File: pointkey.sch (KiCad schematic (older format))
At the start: 12 parts, among them P1 CONN_01X02, SW1 SW_PUSH, SW2 SW_PUSH, U1 4013

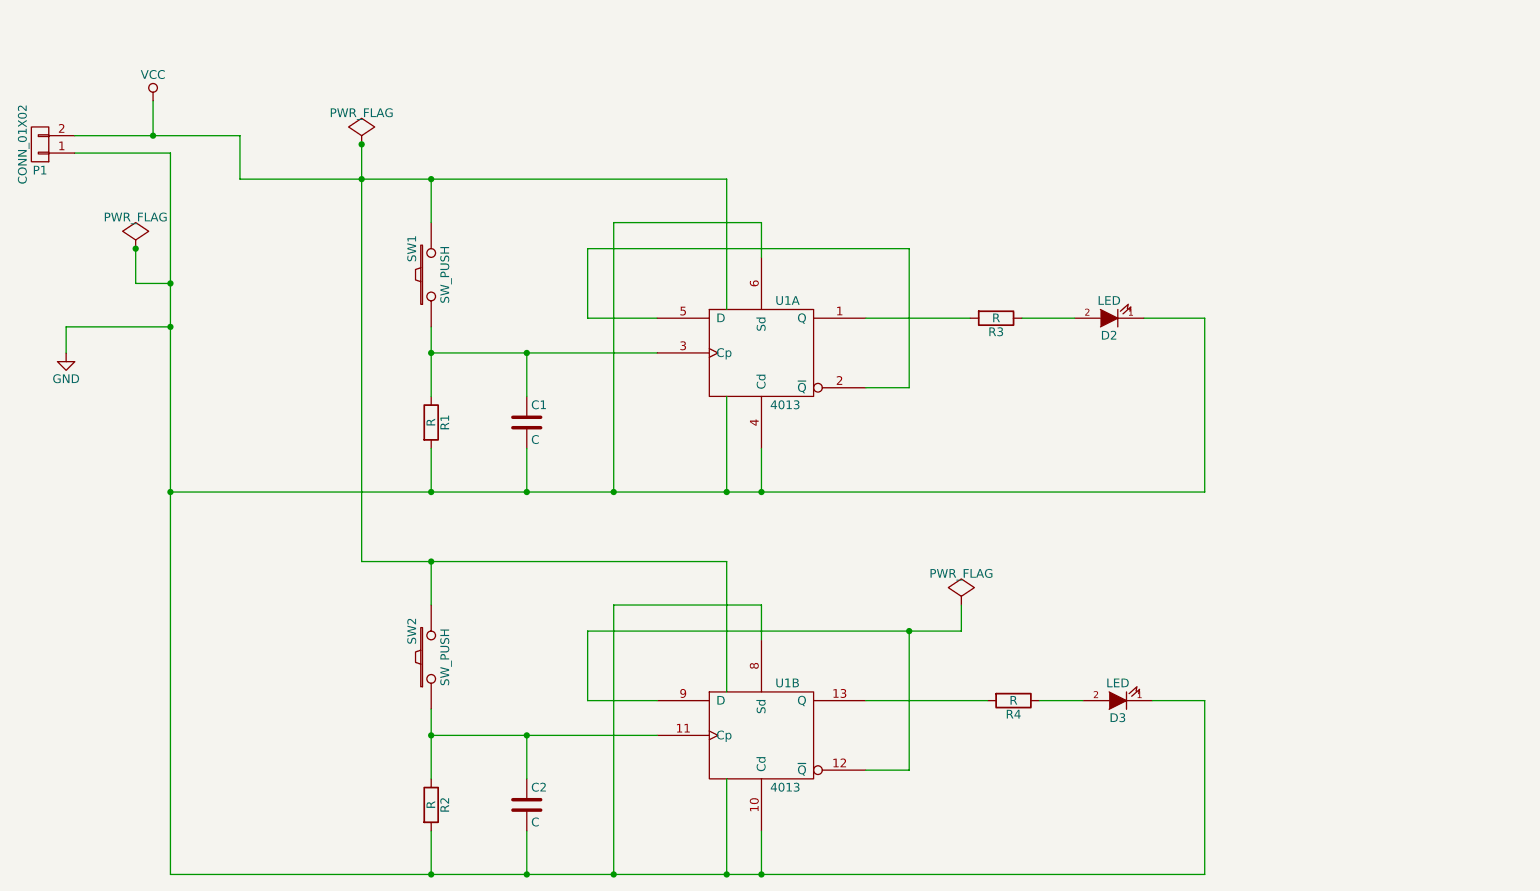
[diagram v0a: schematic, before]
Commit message: debounce
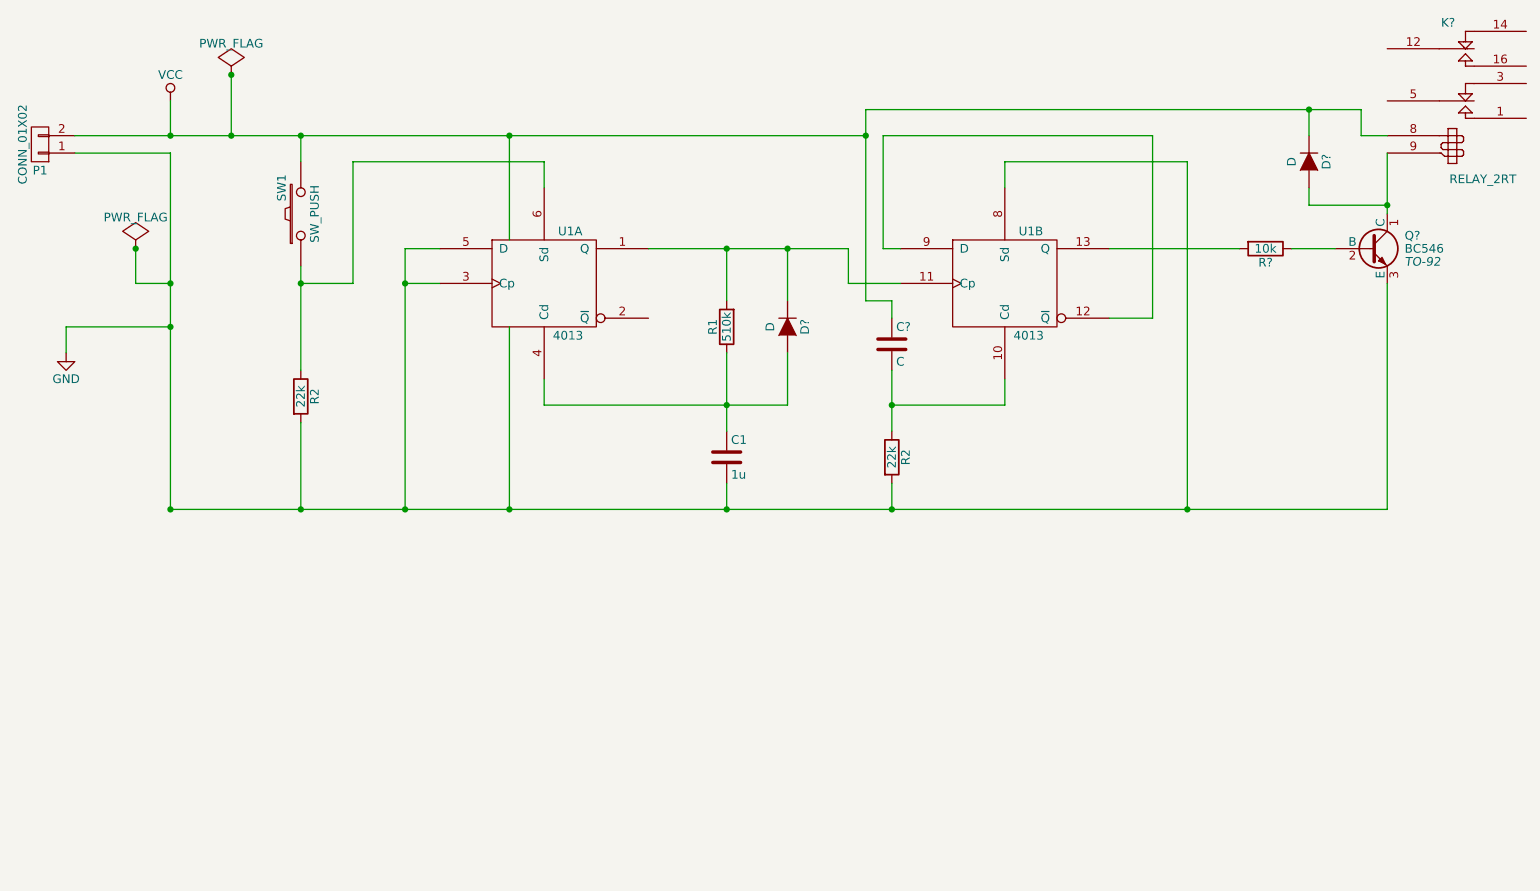
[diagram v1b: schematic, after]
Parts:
- removed C2: C, Capacitors_ThroughHole:C_Radial_D5_L6_P2.5, symbol C
- removed D2, D3: LED, LEDs:LED-3MM, symbol LED
- removed R4: R, Discret:R3-5, symbol R
- removed SW2: SW_PUSH, Buttons_Switches_ThroughHole:SW_PUSH_SMALL, symbol SW_PUSH
- added C?: C, symbol C
- added D? (x2): D, symbol D
- added K?: RELAY_2RT, symbol RELAY_2RT
- added Q?: BC546, TO-92, symbol BC546
- added R?: 10k, symbol R
- C1: value C -> 1u; footprint Capacitors_ThroughHole:C_Radial_D5_L6_P2.5 -> (none)
- R1: renamed from R3; value R -> 510k
- R2: renamed from R1; value R -> 22k
- R2: value R -> 22k; footprint Discret:R3-5 -> (none)
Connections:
- net GND: now also U1.3 (Cp), U1.5 (D), Q?.3 (E); no longer U1.10 (Cd), U1.4 (Cd), U1.6 (Sd)
- net VCC: now also C?.1, D?.1 (K), K?.8
- net at R2.1, SW1.1: now also U1.6 (Sd); no longer C1.1, U1.3 (Cp)
- net at R1.2, U1.1 (Q): now also U1.11 (Cp), D?.1 (K)
- net at U1.2 (~Q): no longer U1.5 (D)
- net at R1.1: now also C1.1, U1.4 (Cd), D?.2 (A)
- net at R2.1: now also U1.10 (Cd), C?.2; no longer U1.11 (Cp)
- net at U1.13 (Q): now also R?.2
- new net: Q?.2 (B), R?.1
- new net: D?.2 (A), K?.9, Q?.1 (C)
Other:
- moved on the sheet: R1, R2, SW1, U1A, U1B
